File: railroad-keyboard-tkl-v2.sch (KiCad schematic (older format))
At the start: 208 parts, among them SW1 SW_Push, U1 ATmega32U4-AU, Y1 16MHz

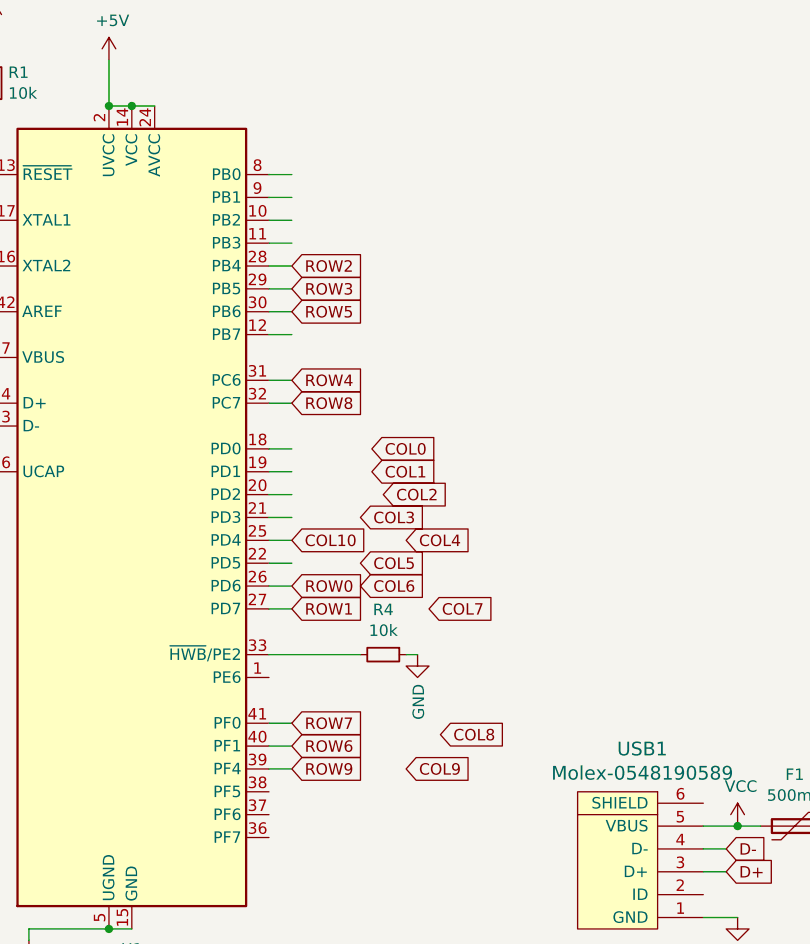
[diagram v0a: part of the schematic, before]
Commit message: Completion of first draft
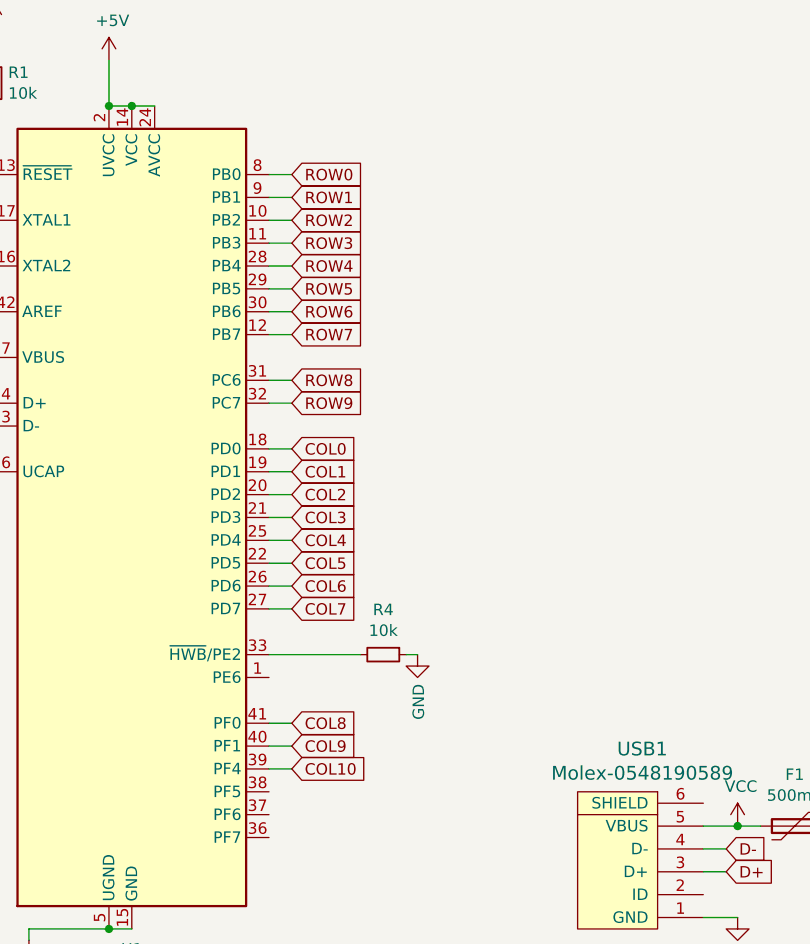
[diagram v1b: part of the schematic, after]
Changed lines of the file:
@@
 Wire Wire Line
 	17000 4350 17000 7350
-Text GLabel 2850 14000 2    50   Input ~ 0
+Text GLabel 2850 12200 2    50   Input ~ 0
 ROW1
-Text GLabel 2850 13900 2    50   Input ~ 0
+Text GLabel 2850 12100 2    50   Input ~ 0
 ROW0
+Text GLabel 2850 12400 2    50   Input ~ 0
+ROW3
+Text GLabel 2850 12300 2    50   Input ~ 0
+ROW2
 Text GLabel 2850 12600 2    50   Input ~ 0
-ROW3
+ROW5
 Text GLabel 2850 12500 2    50   Input ~ 0
-ROW2
+ROW4
+Text GLabel 2850 12800 2    50   Input ~ 0
+ROW7
 Text GLabel 2850 12700 2    50   Input ~ 0
-ROW5
+ROW6
+Text GLabel 2850 13100 2    50   Input ~ 0
+ROW9
 Text GLabel 2850 13000 2    50   Input ~ 0
-ROW4
-Text GLabel 2850 14500 2    50   Input ~ 0
-ROW7
-Text GLabel 2850 14600 2    50   Input ~ 0
-ROW6
-Text GLabel 2850 14700 2    50   Input ~ 0
-ROW9
-Text GLabel 2850 13100 2    50   Input ~ 0
 ROW8
 Wire Wire Line
@@
 Wire Wire Line
 	2850 12200 2750 12200
-Text GLabel 3200 13300 2    50   Input ~ 0
+Text GLabel 2850 13300 2    50   Input ~ 0
 COL0
-Text GLabel 3200 13400 2    50   Input ~ 0
+Text GLabel 2850 13400 2    50   Input ~ 0
 COL1
-Text GLabel 3250 13500 2    50   Input ~ 0
+Text GLabel 2850 13500 2    50   Input ~ 0
 COL2
-Text GLabel 3150 13600 2    50   Input ~ 0
+Text GLabel 2850 13600 2    50   Input ~ 0
 COL3
-Text GLabel 3350 13700 2    50   Input ~ 0
+Text GLabel 2850 13700 2    50   Input ~ 0
 COL4
-Text GLabel 3150 13800 2    50   Input ~ 0
+Text GLabel 2850 13800 2    50   Input ~ 0
 COL5
-Text GLabel 3450 14000 2    50   Input ~ 0
+Text GLabel 2850 14000 2    50   Input ~ 0
 COL7
-Text GLabel 3500 14550 2    50   Input ~ 0
+Text GLabel 2850 14500 2    50   Input ~ 0
 COL8
-Text GLabel 3350 14700 2    50   Input ~ 0
+Text GLabel 2850 14600 2    50   Input ~ 0
 COL9
-Text GLabel 2850 13700 2    50   Input ~ 0
+Text GLabel 2850 14700 2    50   Input ~ 0
 COL10
-Text GLabel 3150 13900 2    50   Input ~ 0
+Text GLabel 2850 13900 2    50   Input ~ 0
 COL6
 Wire Wire Line
